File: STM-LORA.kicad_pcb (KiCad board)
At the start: 2 copper layers, 56.5 x 50.8 mm, 22 parts, among them J1 Batt, J11 CONN_02X09, J13 CONN_01X02, J2 Solar, J3 CONN_01X17, J4 CONN_01X03, J6 CONN_01X01, J9 CONN_01X05, U1 stm32f103c8t6-module-china, U2 RFM95HW

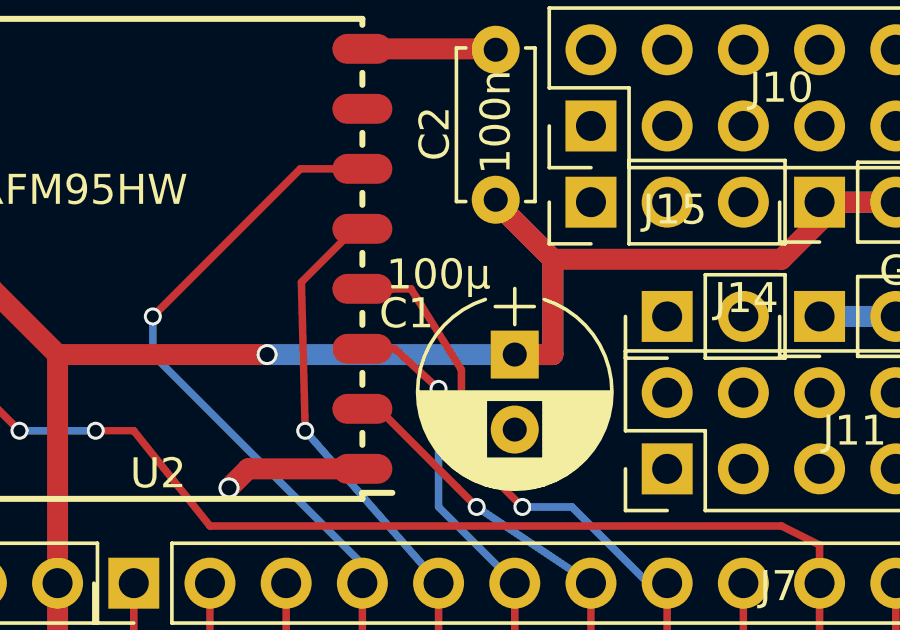
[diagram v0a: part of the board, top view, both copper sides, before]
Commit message: layout silk screen
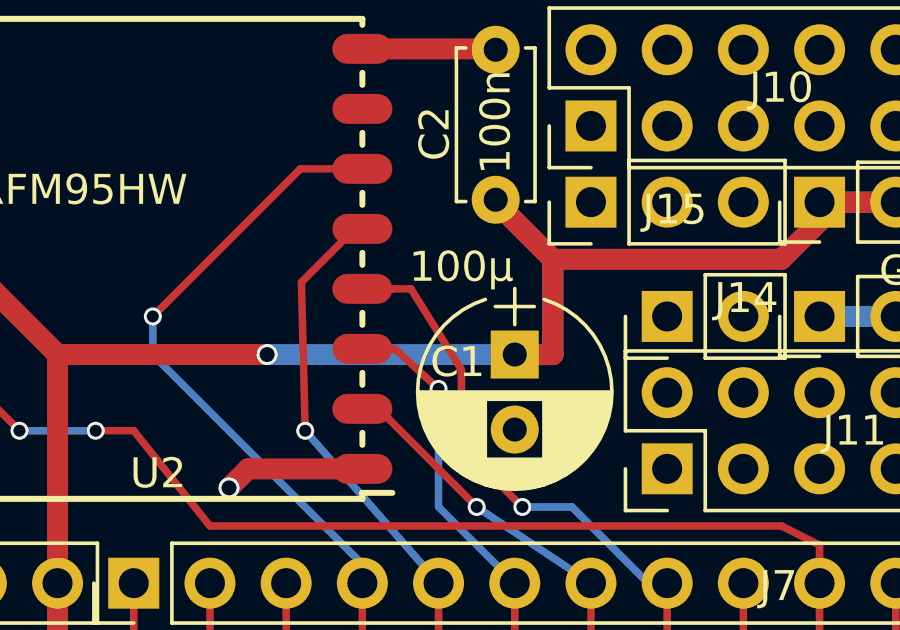
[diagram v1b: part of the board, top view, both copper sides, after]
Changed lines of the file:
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@@
-(kicad_pcb (version 4) (host pcbnew 4.0.6)
+(kicad_pcb (version 4) (host pcbnew 4.0.6-e0-6349~53~ubuntu16.04.1)
   (general
     (links 75)
     (no_connects 0)
-    (area 83.744999 55.563 140.775 109.173333)
+    (area 83.744999 55.804999 140.410001 106.755001)
     (thickness 1.6)
     (drawings 12)
@@
     (descr "CP, Radial series, Radial, pin pitch=2.50mm, , diameter=6.3mm, Electrolytic Capacitor")
     (tags "CP Radial series Radial pin pitch 2.50mm  diameter 6.3mm Electrolytic Capacitor")
-    (fp_text reference C1 (at -1.3716 3.6068 360) (layer F.SilkS)
-      (effects (font (size 1 1) (thickness 0.15)))
-    )
-    (fp_text value 100µ (at -2.667 2.54 360) (layer F.SilkS)
+    (fp_text reference C1 (at 0.254 1.905 360) (layer F.SilkS)
+      (effects (font (size 1 1) (thickness 0.15)))
+    )
+    (fp_text value 100µ (at -2.921 1.778 360) (layer F.SilkS)
       (effects (font (size 1 1) (thickness 0.15)))
     )
@@
     (effects (font (size 1 1) (thickness 0.2)))
   )
-  (segment (start 128.27 67.31) (end 118.11 67.31) (width 0.7) (layer B.Cu) (net 8) (status C00000))
+  (segment (start 128.27 67.31) (end 118.11 67.31) (width 0.7) (layer B.Cu) (net 8))
   (segment (start 130.81 58.42) (end 134.62 58.42) (width 0.7) (layer F.Cu) (net 8) (status 30))
   (segment (start 86.87 60.39) (end 85.155 60.39) (width 0.7) (layer F.Cu) (net 8) (status 10))
